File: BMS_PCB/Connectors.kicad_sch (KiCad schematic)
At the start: 6 parts, among them J1 Conn_01x37

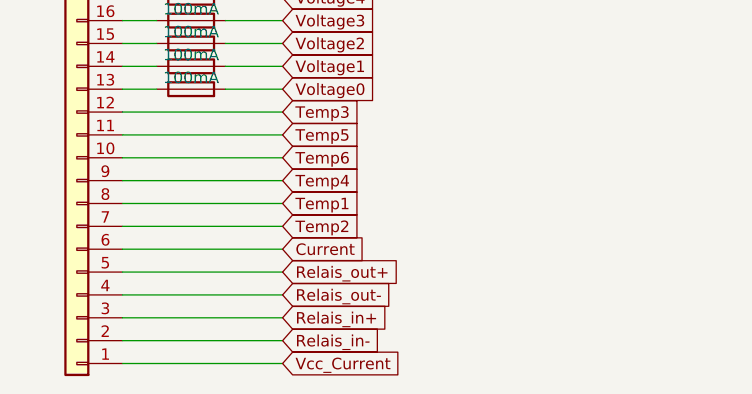
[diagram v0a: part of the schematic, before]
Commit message: Bugfixes
noch ein paar Fehler ausgemerzt
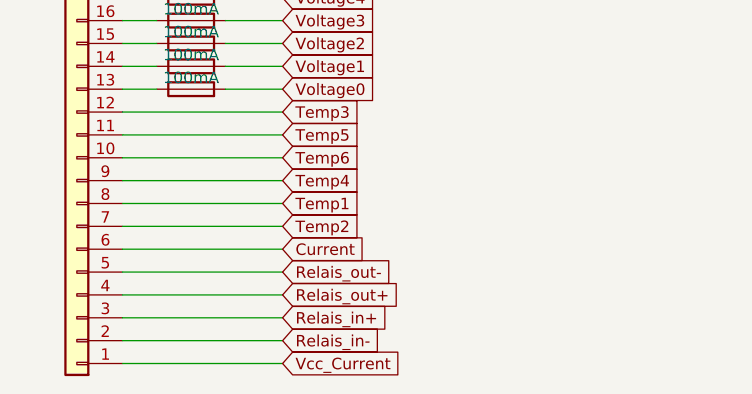
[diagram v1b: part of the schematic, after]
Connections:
- net Relais_out+: now also J1.4 (Pin_4); no longer J1.5 (Pin_5)
- net Relais_out-: now also J1.5 (Pin_5); no longer J1.4 (Pin_4)
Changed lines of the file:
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@@
+	(wire
+		(pts
+			(xy 41.91 85.09) (xy 41.91 87.63)
+		)
+		(stroke
+			(width 0)
+			(type default)
+		)
+	)
+	(wire
+		(pts
+			(xy 36.83 97.79) (xy 41.91 97.79)
+		)
+		(stroke
+			(width 0)
+			(type default)
+		)
+	)
+	(wire
+		(pts
+			(xy 36.83 105.41) (xy 40.64 105.41)
+		)
+		(stroke
+			(width 0)
+			(type default)
+		)
+	)
+	(wire
+		(pts
+			(xy 36.83 138.43) (xy 54.61 138.43)
+		)
+		(stroke
+			(width 0)
+			(type default)
+		)
+	)
+	(wire
+		(pts
+			(xy 36.83 113.03) (xy 40.64 113.03)
+		)
+		(stroke
+			(width 0)
+			(type default)
+		)
+	)
+	(wire
+		(pts
+			(xy 36.83 107.95) (xy 40.64 107.95)
+		)
+		(stroke
+			(width 0)
+			(type default)
+		)
+	)
+	(wire
+		(pts
+			(xy 48.26 113.03) (xy 54.61 113.03)
+		)
+		(stroke
+			(width 0)
+			(type default)
+		)
+	)
+	(wire
+		(pts
+			(xy 36.83 54.61) (xy 39.37 54.61)
+		)
+		(stroke
+			(width 0)
+			(type default)
+		)
+	)
+	(wire
+		(pts
+			(xy 36.83 57.15) (xy 39.37 57.15)
+		)
+		(stroke
+			(width 0)
+			(type default)
+		)
+	)
+	(wire
+		(pts
+			(xy 41.91 92.71) (xy 41.91 95.25)
+		)
+		(stroke
+			(width 0)
+			(type default)
+		)
+	)
+	(wire
+		(pts
+			(xy 36.83 87.63) (xy 41.91 87.63)
+		)
+		(stroke
+			(width 0)
+			(type default)
+		)
+	)
+	(wire
+		(pts
+			(xy 48.26 115.57) (xy 54.61 115.57)
+		)
+		(stroke
+			(width 0)
+			(type default)
+		)
+	)
 	(wire
 		(pts
@@
 	(wire
 		(pts
-			(xy 41.91 85.09) (xy 41.91 87.63)
-		)
-		(stroke
-			(width 0)
-			(type default)
-		)
-	)
-	(wire
-		(pts
-			(xy 36.83 97.79) (xy 41.91 97.79)
-		)
-		(stroke
-			(width 0)
-			(type default)
-		)
-	)
-	(wire
-		(pts
-			(xy 36.83 105.41) (xy 40.64 105.41)
-		)
-		(stroke
-			(width 0)
-			(type default)
-		)
-	)
-	(wire
-		(pts
-			(xy 36.83 113.03) (xy 40.64 113.03)
-		)
-		(stroke
-			(width 0)
-			(type default)
-		)
-	)
-	(wire
-		(pts
-			(xy 36.83 107.95) (xy 40.64 107.95)
-		)
-		(stroke
-			(width 0)
-			(type default)
-		)
-	)
-	(wire
-		(pts
-			(xy 48.26 113.03) (xy 54.61 113.03)
-		)
-		(stroke
-			(width 0)
-			(type default)
-		)
-	)
-	(wire
-		(pts
-			(xy 36.83 54.61) (xy 39.37 54.61)
-		)
-		(stroke
-			(width 0)
-			(type default)
-		)
-	)
-	(wire
-		(pts
-			(xy 36.83 57.15) (xy 39.37 57.15)
-		)
-		(stroke
-			(width 0)
-			(type default)
-		)
-	)
-	(wire
-		(pts
-			(xy 41.91 92.71) (xy 41.91 95.25)
-		)
-		(stroke
-			(width 0)
-			(type default)
-		)
-	)
-	(wire
-		(pts
-			(xy 36.83 87.63) (xy 41.91 87.63)
-		)
-		(stroke
-			(width 0)
-			(type default)
-		)
-	)
-	(wire
-		(pts
-			(xy 48.26 115.57) (xy 54.61 115.57)
-		)
-		(stroke
-			(width 0)
-			(type default)
-		)
-	)
-	(wire
-		(pts
 			(xy 48.26 110.49) (xy 54.61 110.49)
 		)
@@
 	(wire
 		(pts
-			(xy 36.83 138.43) (xy 54.61 138.43)
-		)
-		(stroke
-			(width 0)
-			(type default)
-		)
-	)
-	(wire
-		(pts
 			(xy 36.83 128.27) (xy 54.61 128.27)
 		)
@@
 	(global_label "Relais_out-"
 		(shape input)
+		(at 54.61 135.89 0)
+		(fields_autoplaced yes)
+		(effects
+			(font
+				(size 1.27 1.27)
+			)
+			(justify left)
+		)
+		(property "Intersheetrefs" "${INTERSHEET_REFS}"
+			(at 68.9646 135.89 0)
+			(effects
+				(font
+					(size 1.27 1.27)
+				)
+				(justify left)
+				(hide yes)
+			)
+		)
+	)
+	(global_label "Temp6"
+		(shape input)
+		(at 54.61 123.19 0)
+		(fields_autoplaced yes)
+		(effects
+			(font
+				(size 1.27 1.27)
+			)
+			(justify left)
+		)
+		(property "Intersheetrefs" "${INTERSHEET_REFS}"
+			(at 63.7032 123.19 0)
+			(effects
+				(font
+					(size 1.27 1.27)
+				)
+				(justify left)
+				(hide yes)
+			)
+		)
+	)
+	(global_label "Relais_in-"
+		(shape input)
+		(at 54.61 143.51 0)
+		(fields_autoplaced yes)
+		(effects
+			(font
+				(size 1.27 1.27)
+			)
+			(justify left)
+		)
+		(property "Intersheetrefs" "${INTERSHEET_REFS}"
+			(at 67.6947 143.51 0)
+			(effects
+				(font
+					(size 1.27 1.27)
+				)
+				(justify left)
+				(hide yes)
+			)
+		)
+	)
+	(global_label "Current"
+		(shape input)
+		(at 54.61 133.35 0)
+		(fields_autoplaced yes)
+		(effects
+			(font
+				(size 1.27 1.27)
+			)
+			(justify left)
+		)
+		(property "Intersheetrefs" "${INTERSHEET_REFS}"
+			(at 64.5499 133.35 0)
+			(effects
+				(font
+					(size 1.27 1.27)
+				)
+				(justify left)
+				(hide yes)
+			)
+		)
+	)
+	(global_label "Voltage0"
+		(shape input)
+		(at 54.61 115.57 0)
+		(fields_autoplaced yes)
+		(effects
+			(font
+				(size 1.27 1.27)
+			)
+			(justify left)
+		)
+		(property "Intersheetrefs" "${INTERSHEET_REFS}"
+			(at 65.8198 115.57 0)
+			(effects
+				(font
+					(size 1.27 1.27)
+				)
+				(justify left)
+				(hide yes)
+			)
+		)
+	)
+	(global_label "Relais_out+"
+		(shape input)
 		(at 54.61 138.43 0)
 		(fields_autoplaced yes)
@@
 			(effects
 				(font
-					(size 1.27 1.27)
-				)
-				(justify left)
-				(hide yes)
-			)
-		)
-	)
-	(global_label "Temp6"
-		(shape input)
-		(at 54.61 123.19 0)
-		(fields_autoplaced yes)
-		(effects
-			(font
-				(size 1.27 1.27)
-			)
-			(justify left)
-		)
-		(property "Intersheetrefs" "${INTERSHEET_REFS}"
-			(at 63.7032 123.19 0)
-			(effects
-				(font
-					(size 1.27 1.27)
-				)
-				(justify left)
-				(hide yes)
-			)
-		)
-	)
-	(global_label "Relais_in-"
-		(shape input)
-		(at 54.61 143.51 0)
-		(fields_autoplaced yes)
-		(effects
-			(font
-				(size 1.27 1.27)
-			)
-			(justify left)
-		)
-		(property "Intersheetrefs" "${INTERSHEET_REFS}"
-			(at 67.6947 143.51 0)
-			(effects
-				(font
-					(size 1.27 1.27)
-				)
-				(justify left)
-				(hide yes)
-			)
-		)
-	)
-	(global_label "Current"
-		(shape input)
-		(at 54.61 133.35 0)
-		(fields_autoplaced yes)
-		(effects
-			(font
-				(size 1.27 1.27)
-			)
-			(justify left)
-		)
-		(property "Intersheetrefs" "${INTERSHEET_REFS}"
-			(at 64.5499 133.35 0)
-			(effects
-				(font
-					(size 1.27 1.27)
-				)
-				(justify left)
-				(hide yes)
-			)
-		)
-	)
-	(global_label "Voltage0"
-		(shape input)
-		(at 54.61 115.57 0)
-		(fields_autoplaced yes)
-		(effects
-			(font
-				(size 1.27 1.27)
-			)
-			(justify left)
-		)
-		(property "Intersheetrefs" "${INTERSHEET_REFS}"
-			(at 65.8198 115.57 0)
-			(effects
-				(font
-					(size 1.27 1.27)
-				)
-				(justify left)
-				(hide yes)
-			)
-		)
-	)
-	(global_label "Relais_out+"
-		(shape input)
-		(at 54.61 135.89 0)
-		(fields_autoplaced yes)
-		(effects
-			(font
-				(size 1.27 1.27)
-			)
-			(justify left)
-		)
-		(property "Intersheetrefs" "${INTERSHEET_REFS}"
-			(at 68.9646 135.89 0)
-			(effects
-				(font
